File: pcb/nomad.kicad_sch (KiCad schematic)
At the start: 38 parts, among them J1 USB_C_Receptacle_USB2.0_16P, SW1 UP, SW2 DOWN, SW3 RIGHT, SW4 LEFT, SW5 SEL, SW6 SW_Push, SW7 SW_Push, U1 ESP32-S3-WROOM-1, U2 PCF8574T, U3 MAX17048G_T10, U5 CH343G, U7 AMS1117-3.3, U8 BQ24075RGT

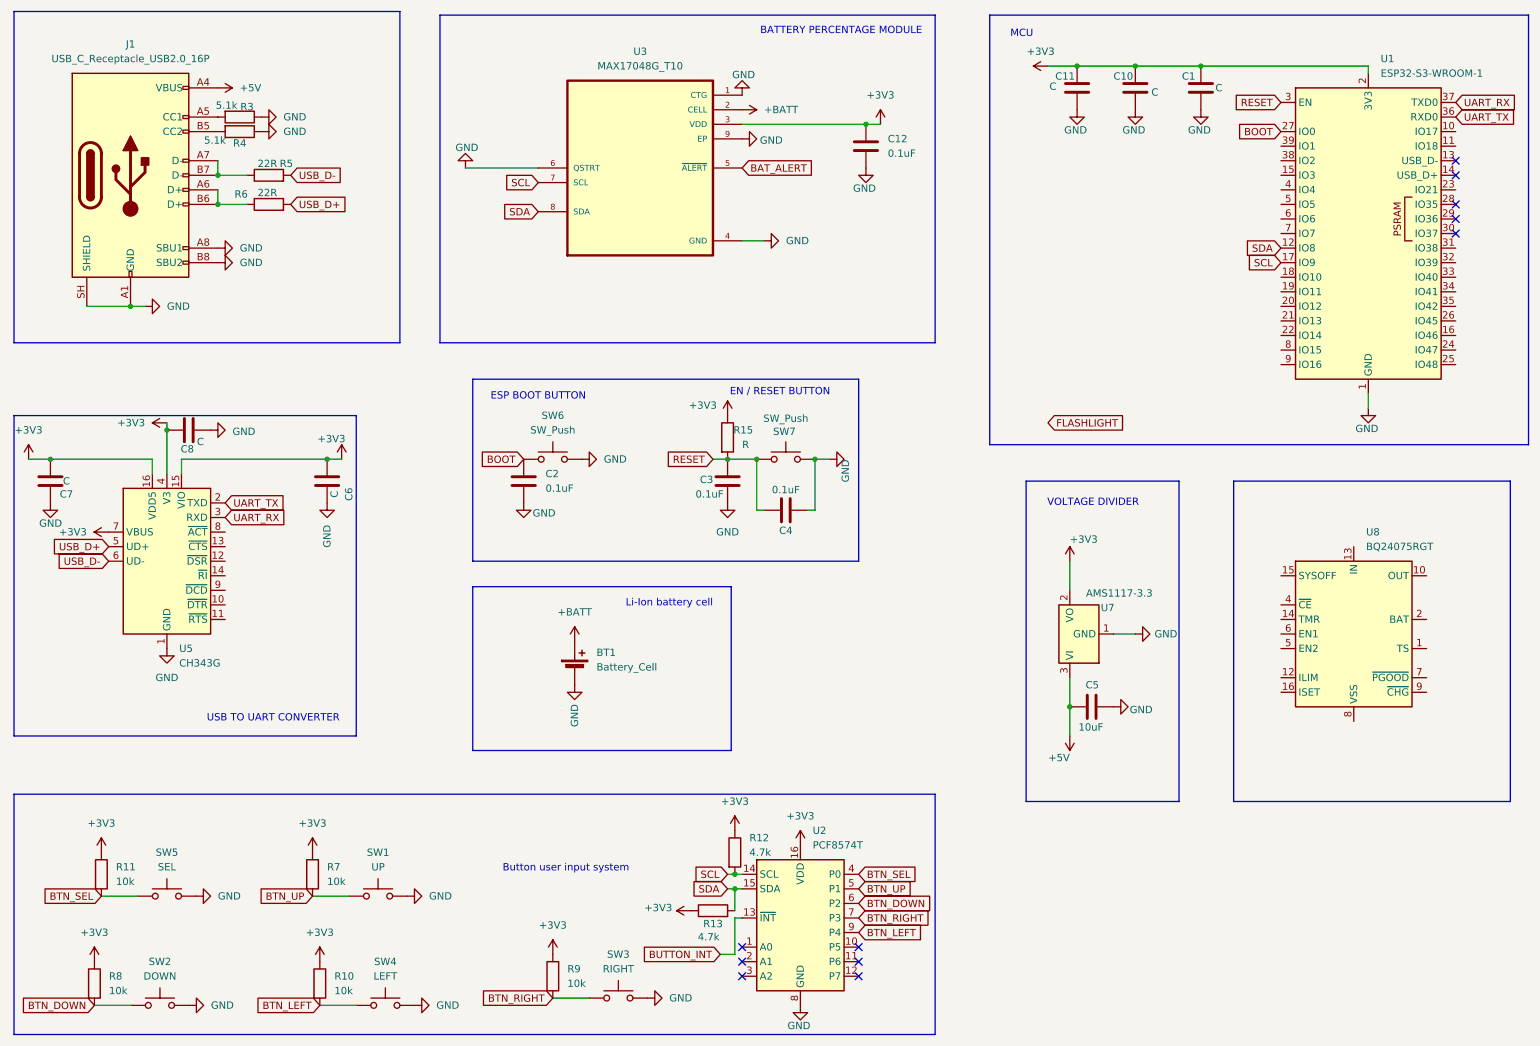
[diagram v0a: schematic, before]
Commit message: Updating PCB
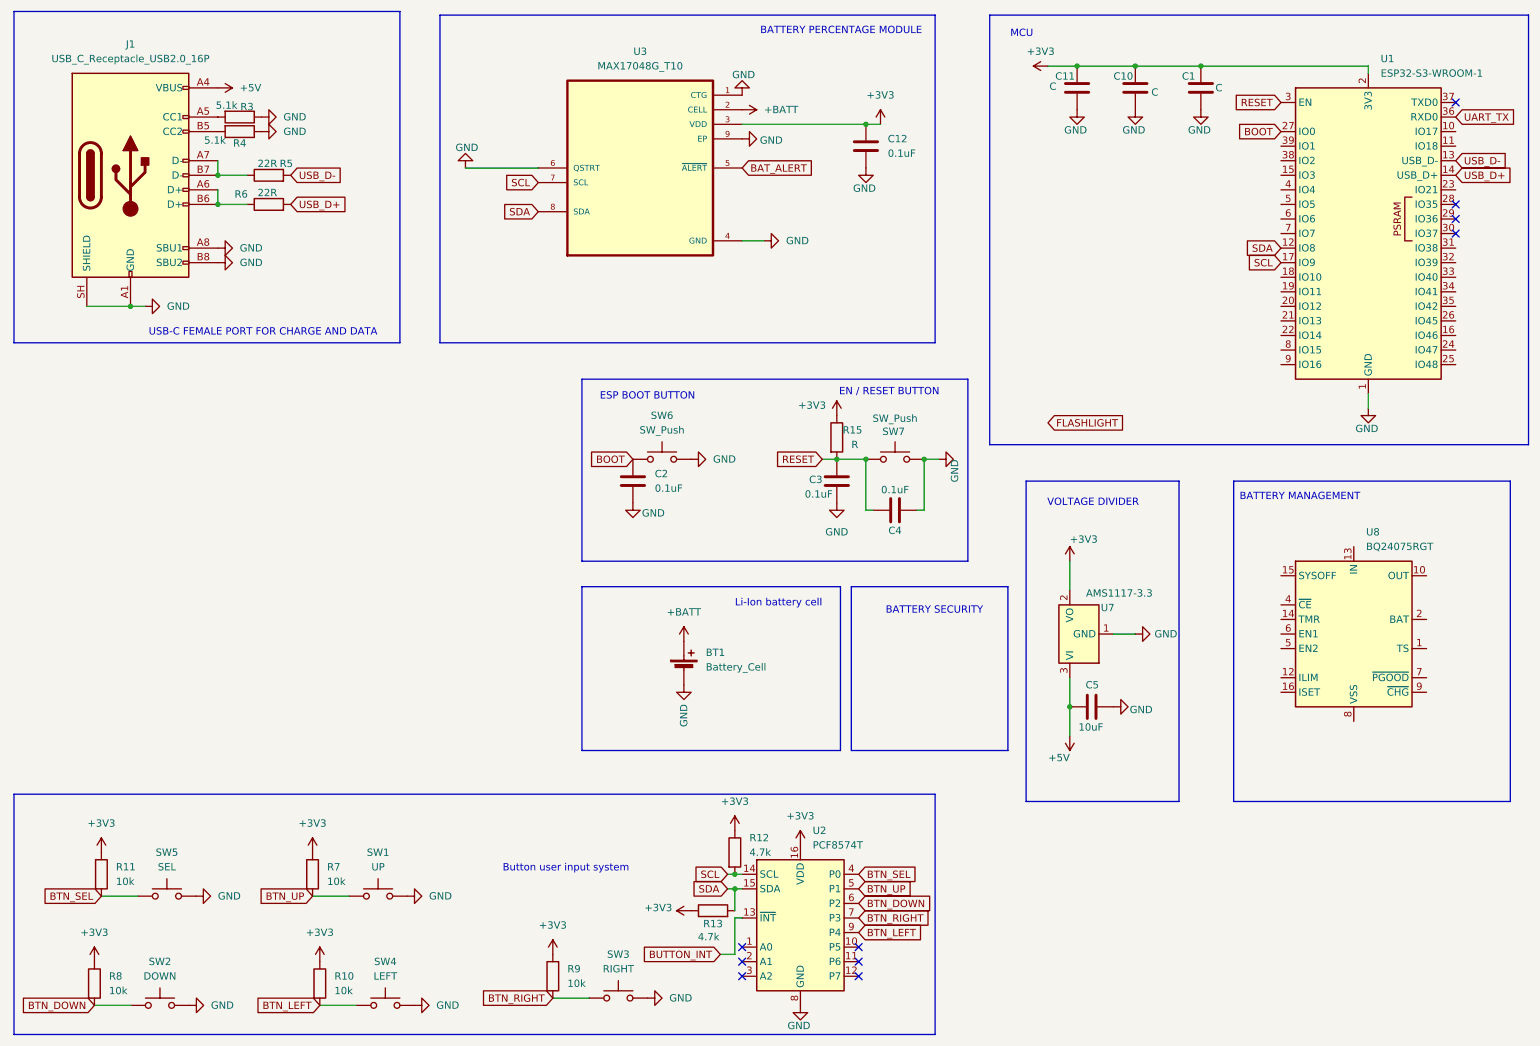
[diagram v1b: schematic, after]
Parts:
- removed C6, C7, C8: C, Capacitor_SMD:C_0805_2012Metric, symbol Device:C
- removed U5: CH343G, Package_SO:SOIC-16_3.9x9.9mm_P1.27mm, symbol Interface_USB:CH343G
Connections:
- net USB_D+: now also U1.14 (USB_D+)
- net USB_D-: now also U1.13 (USB_D-)
- net UART_RX: no longer names the net of U1.37 (TXD0)
- no-connect marks 11 -> 10
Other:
- note added: "BATTERY MANAGEMENT"
- note added: "BATTERY SECURITY"
- note added: "USB-C FEMALE PORT FOR CHARGE AND DATA"
- note removed: "USB TO UART CONVERTER"
- moved on the sheet: BT1, C2, C3, C4, R15, SW6, SW7
